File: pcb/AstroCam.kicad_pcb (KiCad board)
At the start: 2 copper layers, 50 x 50 mm, 0 parts

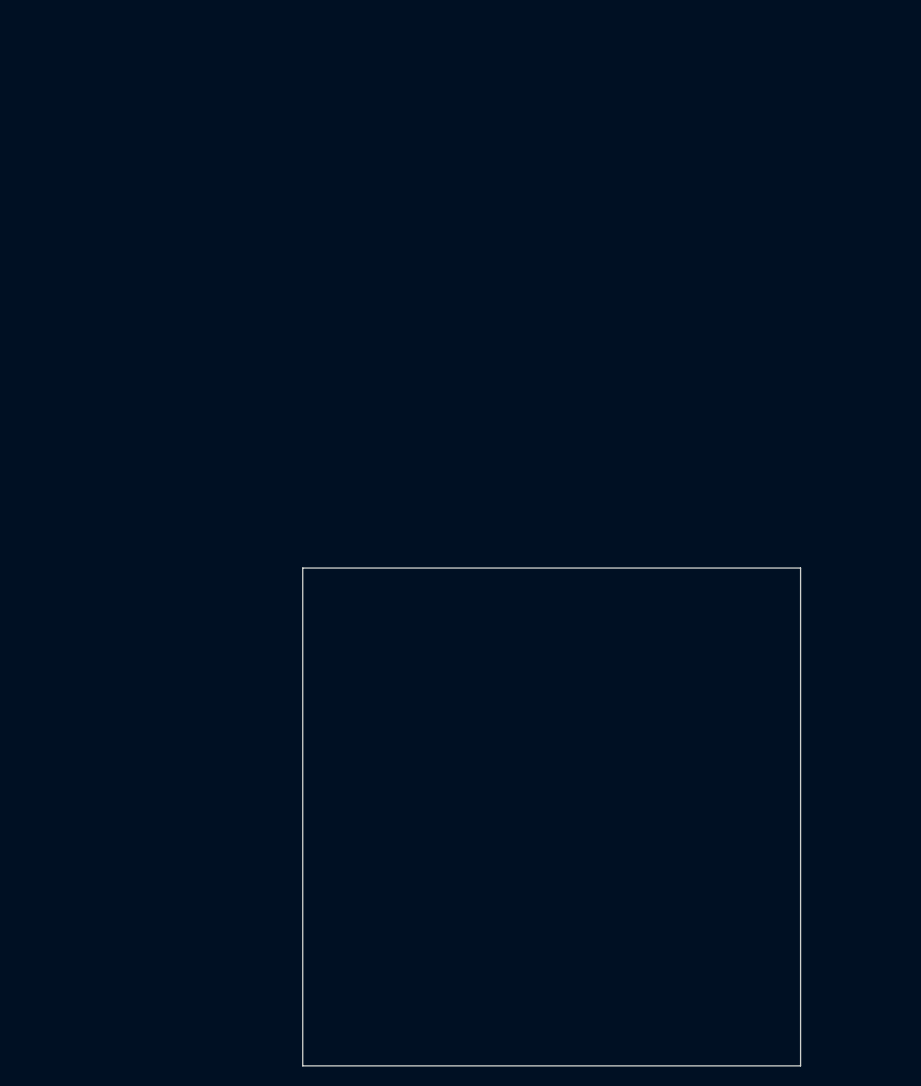
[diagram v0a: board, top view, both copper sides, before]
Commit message: lastest at home
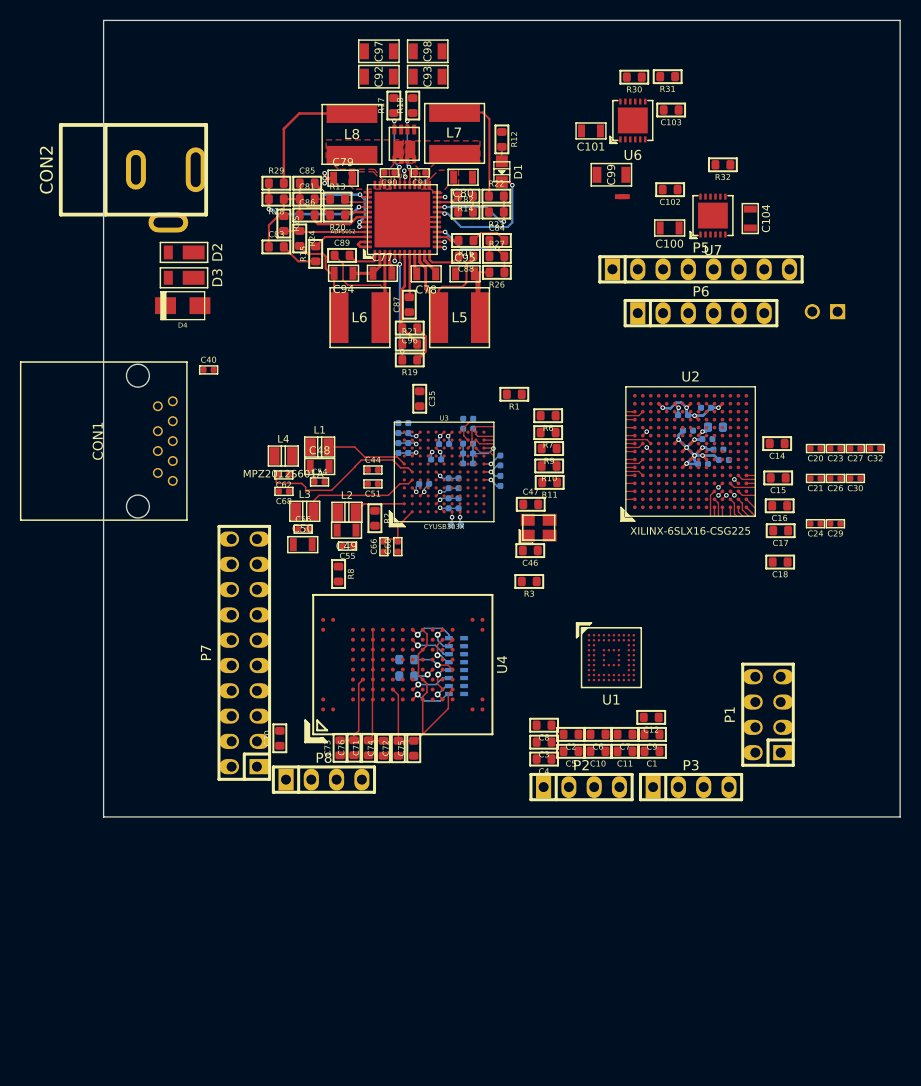
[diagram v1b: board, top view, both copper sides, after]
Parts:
- added C1: 4.7uF, engstad:C0603, F.Cu at (100.1, 118.4)
- added C10: 0.1uF, engstad:C0603, F.Cu at (94.7, 118.4)
- added C100: 1uF, engstad:0805, F.Cu at (101.8, 65.8)
- added C101: 10nF, engstad:0805, F.Cu at (94.0, 56.1)
- added C102: 10nF, engstad:C0603, F.Cu at (101.9, 62.0)
- added C103: 10uF, engstad:C0603, F.Cu at (102.0, 54.0)
- added C104: 10uF, engstad:0805, F.Cu at (110.0, 64.9)
- added C11: 0.1u, engstad:C0603, F.Cu at (97.4, 118.4)
- added C12: 0.1u, engstad:C0603, F.Cu at (100.0, 115.0)
- added C13: 4.7uF, engstad:C0603, B.Cu at (106.5, 85.8)
- added C14: 100uF, engstad:C0603, F.Cu at (112.7, 87.5)
- added C15: 100uF, engstad:C0603, F.Cu at (112.8, 91.0)
- added C16: 100uF, engstad:C0603, F.Cu at (112.9, 93.8)
- added C17: 100uF, engstad:C0603, F.Cu at (113.0, 96.2)
- added C18: 100uF, engstad:C0603, F.Cu at (113.0, 99.4)
- added C19: 4.7uF, engstad:0402, B.Cu at (105.7, 87.0)
- added C2: 0.1uF, engstad:C0603, F.Cu at (91.9, 116.7)
- added C20: 4.7uF, engstad:0402, F.Cu at (116.5, 88.0)
- added C21: 4.7uF, engstad:0402, F.Cu at (116.5, 91.0)
- added C22: 4.7uF, engstad:0402, B.Cu at (105.5, 83.9)
- added C23: 4.7uF, engstad:0402, F.Cu at (118.5, 88.0)
- added C24: 4.7uF, engstad:0402, F.Cu at (116.5, 95.5)
- added C25: 4.7uF, engstad:0402, B.Cu at (106.8, 88.1)
- added C26: .47uF, engstad:0402, F.Cu at (118.5, 91.0)
- added C27: .47uF, engstad:0402, F.Cu at (120.5, 88.0)
- added C28: .47uF, engstad:0402, B.Cu at (103.2, 84.7)
- added C29: .47uF, engstad:0402, F.Cu at (118.5, 95.5)
- added C3: 0.1uF, engstad:C0603, F.Cu at (89.2, 117.5)
- added C30: .47uF, engstad:0402, F.Cu at (120.5, 91.0)
- added C31: 4.7uF, engstad:0402, B.Cu at (107.3, 89.2)
- added C32: .47uF, engstad:0402, F.Cu at (122.5, 88.0)
- added C33: 4.7uF, engstad:0402, B.Cu at (103.7, 86.2)
- added C34: .47uF, engstad:0402, B.Cu at (105.2, 89.5)
- added C35: 22uF, engstad:C0603, F.Cu at (76.8, 83.0)
- added C36: 0.1uF, engstad:0402, B.Cu at (75.6, 88.0)
- added C37: 10nF, engstad:0402, B.Cu at (74.6, 88.0)
- added C38: 0.1uF, engstad:0402, B.Cu at (81.6, 86.0)
- added C39: 10nF, engstad:0402, B.Cu at (81.6, 85.0)
- added C4: 0.1uF, engstad:C0603, F.Cu at (89.2, 119.2)
- added C40: 0.1uF, engstad:0402, F.Cu at (55.5, 80.1)
- added C41: 0.1uF, engstad:0402, B.Cu at (84.8, 91.2)
- added C42: 0.1uF, engstad:0402, B.Cu at (79.2, 87.5)
- added C43: 10nF, engstad:0402, B.Cu at (78.4, 89.1)
- added C44: 0.1uF, engstad:0402, F.Cu at (72.0, 90.2)
- added C45: 0.1uF, engstad:0402, B.Cu at (84.8, 89.2)
- added C46: 12pF, engstad:C0603, F.Cu at (87.8, 98.2)
- added C47: 12pF, engstad:C0603, F.Cu at (87.9, 93.6)
- added C48: 2.2uF, engstad:0805, F.Cu at (66.7, 89.8)
- added C49: 22uF, engstad:0805, F.Cu at (69.4, 96.2)
- added C5: 0.1uF, engstad:C0603, F.Cu at (91.9, 118.4)
- added C50: 22uF, engstad:0805, F.Cu at (65.0, 97.7)
- added C51: 0.1uF, engstad:0402, F.Cu at (72.0, 91.5)
- added C52: 10nF, engstad:0402, B.Cu at (77.2, 91.5)
- added C53: 0.1uF, engstad:0402, B.Cu at (80.4, 95.7)
- added C54: 0.1uF, engstad:0402, F.Cu at (66.7, 91.3)
- added C55: 0.1uF, engstad:0402, F.Cu at (69.5, 97.8)
- added C56: 0.1uF, engstad:0402, F.Cu at (65.0, 96.1)
- added C57: 100nF, engstad:0402, B.Cu at (81.6, 89.5)
- added C58: 100nF, engstad:0402, B.Cu at (80.7, 93.5)
- added C59: 100nF, engstad:0402, B.Cu at (80.7, 91.5)
- added C6: 0.1uF, engstad:C0603, F.Cu at (94.7, 116.7)
- added C60: 100nF, engstad:0402, F.Cu at (74.5, 97.8)
- added C61: 100nF, engstad:0402, B.Cu at (74.6, 85.9)
- added C62: 100nF, engstad:0402, F.Cu at (63.1, 90.7)
- added C63: 100nF, engstad:0402, B.Cu at (81.6, 88.5)
- added C64: 10nF, engstad:0402, B.Cu at (79.7, 93.5)
- added C65: 10nF, engstad:0402, B.Cu at (79.7, 91.5)
- added C66: 10nF, engstad:0402, F.Cu at (73.2, 97.8)
- added C67: 10nF, engstad:0402, B.Cu at (75.6, 85.9)
- added C68: 10nF, engstad:0402, F.Cu at (63.1, 92.3)
- added C69: 10nF, engstad:0402, B.Cu at (81.6, 87.5)
- added C7: 0.1uF, engstad:C0603, F.Cu at (97.4, 116.7)
- added C70: 0.1uF, engstad:C0603, F.Cu at (62.7, 117.1)
- added C71: 100nF, engstad:C0603, F.Cu at (71.6, 118.1)
- added C72: 100nF, engstad:C0603, F.Cu at (74.6, 118.1)
- added C73: 100nF, engstad:C0603, F.Cu at (68.8, 118.1)
- added C74: 2.2uF, engstad:C0603, F.Cu at (73.1, 118.1)
- added C75: 2.2uF, engstad:C0603, F.Cu at (76.2, 118.1)
- added C76: 1.0uF, engstad:C0603, F.Cu at (70.2, 118.0)
- added C77: 10uF/25V, engstad:0805, F.Cu at (73.0, 70.4)
- added C78: 10uF/25V, engstad:0805, F.Cu at (77.4, 70.5)
- added C79: 10uF/25V, engstad:0805, F.Cu at (69.0, 60.9)
- added C8: 0.1uF, engstad:C0603, F.Cu at (89.2, 115.8)
- added C80: 10uF/25V, engstad:0805, F.Cu at (81.1, 60.8)
- added C81: 2.7nF, engstad:C0603, F.Cu at (65.5, 63.0)
- added C82: 2.7nF, engstad:C0603, F.Cu at (81.3, 64.2)
- added C83: 2.7nF, engstad:C0603, F.Cu at (62.4, 67.8)
- added C84: 2.7nF, engstad:C0603, F.Cu at (84.5, 67.1)
- added C85: 1.0uF, engstad:C0603, F.Cu at (65.5, 61.4)
- added C86: 1.0uF, engstad:C0603, F.Cu at (65.5, 64.5)
- added C87: 1uF, engstad:C0603, F.Cu at (75.7, 73.5)
- added C88: 0.1uF, engstad:C0603, F.Cu at (81.4, 68.7)
- added C89: 0.1uF, engstad:C0603, F.Cu at (69.0, 68.6)
- added C9: 0.1uF, engstad:C0603, F.Cu at (100.1, 116.7)
- added C90: 0.1uF, engstad:0402, F.Cu at (73.7, 60.3)
- added C91: 0.1uF, engstad:0402, F.Cu at (76.8, 60.3)
- added C92: 47uF, engstad:1206, F.Cu at (72.7, 50.6)
- added C93: 47uF, engstad:1206, F.Cu at (77.5, 50.6)
- added C94: 22uF, engstad:0805, F.Cu at (69.1, 70.4)
- added C95: 22uF, engstad:0805, F.Cu at (81.3, 70.5)
- added C96: 1.0uF, engstad:C0603, F.Cu at (75.8, 75.9)
- added C97: 47uF, engstad:1206, F.Cu at (72.7, 48.1)
- added C98: 47uF, engstad:1206, F.Cu at (77.5, 48.1)
- added C99: 1uF, engstad:1206, F.Cu at (96.0, 60.5)
- added CON1: USB3, engstad:conn-usb-3.0-fci, F.Cu at (48.5, 87.2)
- added CON2: BARREL_JACK, w_conn_misc:dc_socket, F.Cu at (48.0, 60.0)
- added D1: LED, w_smd_leds:Led_0805, F.Cu at (85.0, 60.2)
- added D2: D_Schottky, engstad:diode-smd-powerdi-123, F.Cu at (53.0, 68.3)
- added D3: D_Schottky, engstad:diode-smd-powerdi-123, F.Cu at (53.0, 70.8)
- added D4: 15V, w_smd_diode:do214ac, F.Cu at (53.0, 73.7)
- added JP1: Jumper_NO_Small, engstad:pin-socket-2, F.Cu at (117.5, 74.2)
- added L1: MPZ2012S601A, w_smd_inductors:inductor_smd_0805, F.Cu at (66.7, 87.8)
- added L2: MPZ2012S601A, w_smd_inductors:inductor_smd_0805, F.Cu at (69.4, 94.4)
- added L3: MPZ2012S601A, w_smd_inductors:inductor_smd_0805, F.Cu at (65.2, 94.3)
- added L4: MPZ2012S601A, w_smd_inductors:inductor_smd_0805, F.Cu at (63.0, 88.8)
- added L5: 10uH, engstad:inductor-smd-60x60, F.Cu at (80.8, 74.8)
- added L6: 4.7uH, engstad:inductor-smd-60x60, F.Cu at (70.8, 74.8)
- added L7: 3.3uH, engstad:inductor-smd-60x60, F.Cu at (80.2, 56.4)
- added L8: 2.2uH, engstad:inductor-smd-60x60, F.Cu at (70.0, 56.5)
- added P1: CONN_02X04, w_pin_strip:pin_strip_4x2, F.Cu at (111.7, 114.7)
- added P2: CONN_01X04, w_pin_strip:pin_strip_4, F.Cu at (93.0, 122.0)
- added P3: CONN_01X04, w_pin_strip:pin_strip_4, F.Cu at (104.0, 122.0)
- added P5: VDRV, w_pin_strip:pin_strip_8, F.Cu at (105.0, 70.0)
- added P6: HDRV, w_pin_strip:pin_strip_6, F.Cu at (105.0, 74.4)
- added P7: CONN_02X10, w_pin_strip:pin_socket_10x2, F.Cu at (59.1, 108.5)
- added P8: UART, w_pin_strip:pin_socket_4, F.Cu at (67.1, 121.2)
- added Q1: Si7232DN, engstad:smd-powerpak-1212-8-dual, F.Cu at (75.2, 57.4)
- added R1: 6K04/1%, engstad:R0603, F.Cu at (86.2, 82.5)
- added R10: 4K7, engstad:R0603, F.Cu at (89.8, 89.8)
- added R11: 330R, engstad:R0603, F.Cu at (89.8, 91.4)
- added R12: 220, engstad:R0603, F.Cu at (85.0, 57.0)
- added R13: 10.0k, engstad:R0603, F.Cu at (68.5, 63.0)
- added R14: 15.0k, engstad:R0603, F.Cu at (81.3, 62.6)
- added R15: 6.81k, engstad:R0603, F.Cu at (66.3, 68.5)
- added R16: 6.81k, engstad:R0603, F.Cu at (81.4, 67.1)
- added R17: 22k, engstad:R0603, F.Cu at (74.2, 53.5)
- added R18: 22k, engstad:R0603, F.Cu at (76.0, 53.5)
- added R19: 10.0k, engstad:R0603, F.Cu at (75.8, 79.1)
- added R2: 200R/1%, engstad:R0603, F.Cu at (72.2, 95.0)
- added R20: 31.6k, engstad:R0603, F.Cu at (68.5, 64.5)
- added R21: 26.7k, engstad:R0603, F.Cu at (75.8, 77.5)
- added R22: 31.6k, engstad:R0603, F.Cu at (84.5, 62.6)
- added R23: 10.2k, engstad:R0603, F.Cu at (84.5, 64.2)
- added R24: 4.99k, engstad:R0603, F.Cu at (64.7, 66.9)
- added R25: 10.0k, engstad:R0603, F.Cu at (63.1, 65.4)
- added R26: 59.0k, engstad:R0603, F.Cu at (84.5, 70.3)
- added R27: 10.0k, engstad:R0603, F.Cu at (84.5, 68.7)
- added R28: 10.2k, engstad:R0603, F.Cu at (62.4, 63.0)
- added R29: 12.7k, engstad:R0603, F.Cu at (62.4, 61.4)
- added R3: 22R, engstad:R0603, F.Cu at (87.8, 101.3)
- added R30: 23.2K, engstad:R0603, F.Cu at (98.3, 50.7)
- added R31: 13.3K, engstad:R0603, F.Cu at (101.7, 50.6)
- added R32: 15.0K, engstad:R0603, F.Cu at (107.2, 59.5)
- added R4: 49K9, engstad:R0603, B.Cu at (75.5, 110.8)
- added R5: 49K9, engstad:R0603, B.Cu at (75.5, 109.2)
- added R6: 4K7, engstad:R0603, F.Cu at (89.7, 84.7)
- added R7: 4K7, engstad:R0603, F.Cu at (89.7, 86.4)
- added R8: 47K, engstad:R0603, F.Cu at (68.6, 100.6)
- added R9: 4K7, engstad:R0603, F.Cu at (89.8, 88.0)
- added RP1: 49K9, w_smd_resistors:r_cat16-8, B.Cu at (80.4, 109.8)
- added T1: NET-TIE, engstad:net-tie-0.5mm, F.Cu at (97.1, 62.7)
- added U1: ADDI7013, engstad:csp-bga-bc-76-3, F.Cu at (96.0, 109.0)
- added U2: XILINX-6SLX16-CSG225, engstad:csg225, F.Cu at (104.0, 88.3)
- added U3: CYUSB303X, w_smd_bga:xbga121-std, F.Cu at (79.2, 90.3)
- added U4: MTFC4GLDDQ-4M IT, engstad:lfbga-100, F.Cu at (75.0, 109.7)
- added U5: ADP5052, w_smd_qfn:pvqfn-n48, F.Cu at (75.0, 65.0)
- added U6: LP38798, engstad:wson-12, F.Cu at (98.2, 55.0)
- added U7: LP38798, engstad:wson-12, F.Cu at (106.2, 64.6)
- added Y1: 19.2 MHz, engstad:crystal-32x25, F.Cu at (88.7, 96.0)
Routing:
- net +3V3: track 0.00 -> 73.3 mm, vias 0 -> 6
- net GND: track 0.00 -> 58.6 mm, vias 0 -> 18
- net +1V2: track 0.00 -> 29.0 mm, vias 0 -> 8
- net /usb-ctrl/CVDD: track 0.00 -> 16.9 mm
- net /power/SW3: track 0.00 -> 16.6 mm
- net /power/VREG: track 0.00 -> 16.2 mm, vias 0 -> 7
- net /power/SW4: track 0.00 -> 16.0 mm
- net /power/PWRGD: track 0.00 -> 13.3 mm, vias 0 -> 2
- net /power/FB1: track 0.00 -> 13.0 mm, vias 0 -> 2
- net +1V8: track 0.00 -> 12.9 mm
- net /usb-ctrl/VDD_1.2V: track 0.00 -> 12.0 mm, vias 0 -> 7
- net /usb-ctrl/TXVDD: track 0.00 -> 11.8 mm
- net /power/FB5: track 0.00 -> 11.6 mm, vias 0 -> 2
- net /power/FB2: track 0.00 -> 9.88 mm, vias 0 -> 2
- net 1V8A: track 0.00 -> 9.74 mm
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- added copper zone on F.Cu, net /power/PVIN
- added copper zone on F.Cu, net /power/SW1
- added copper zone on F.Cu, net /power/SW2
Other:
- board size 50 x 50 mm -> 80 x 80 mm
- copper layers 2 -> 4
